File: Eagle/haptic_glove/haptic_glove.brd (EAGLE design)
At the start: 100 x 80 mm, 58 parts, among them U1 DRV2605L, U2 DRV2605L, U3 DRV2605L, U4 DRV2605L, U5 MPU-6050-1, U6 MCP73833, X1 TSW-121-07-G-S, X2 TSW-121-07-G-S, X3 TSW-121-07-G-S, X4 TSW-121-07-G-S

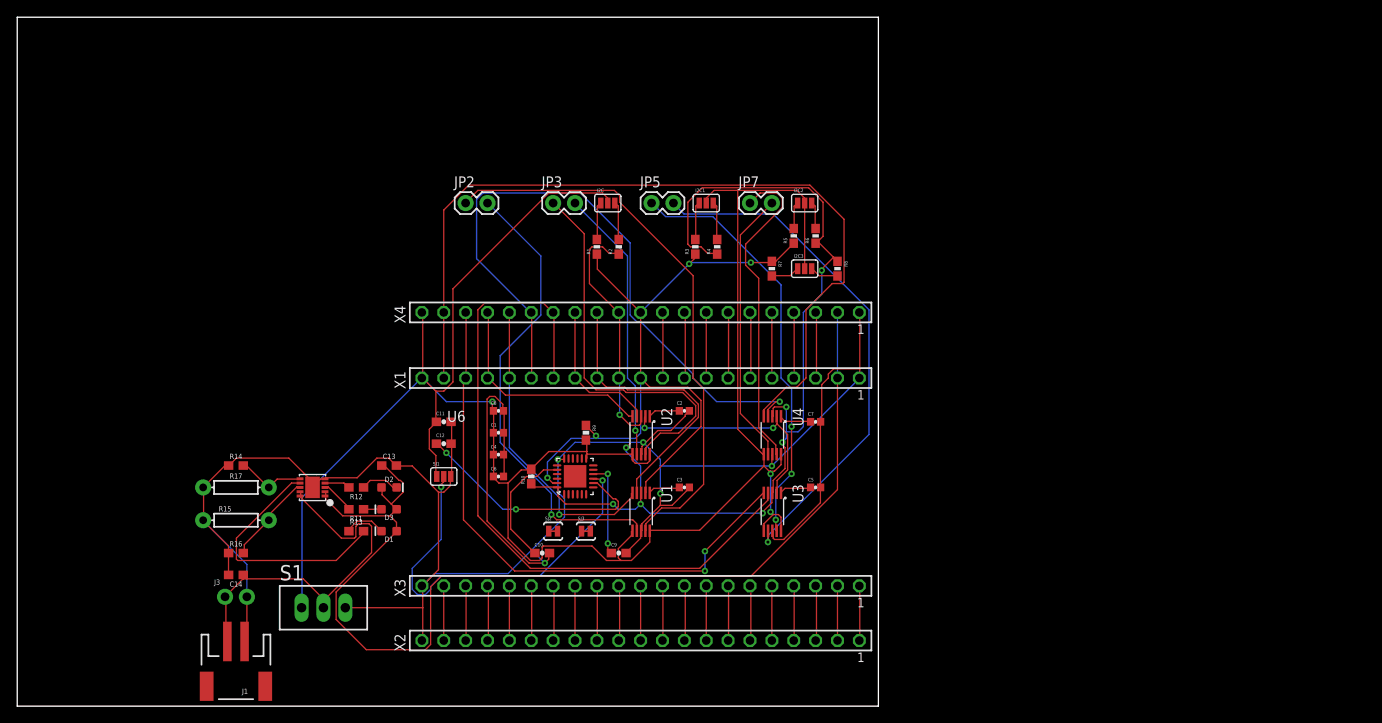
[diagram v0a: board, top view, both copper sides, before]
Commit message: Updated schematic and board design
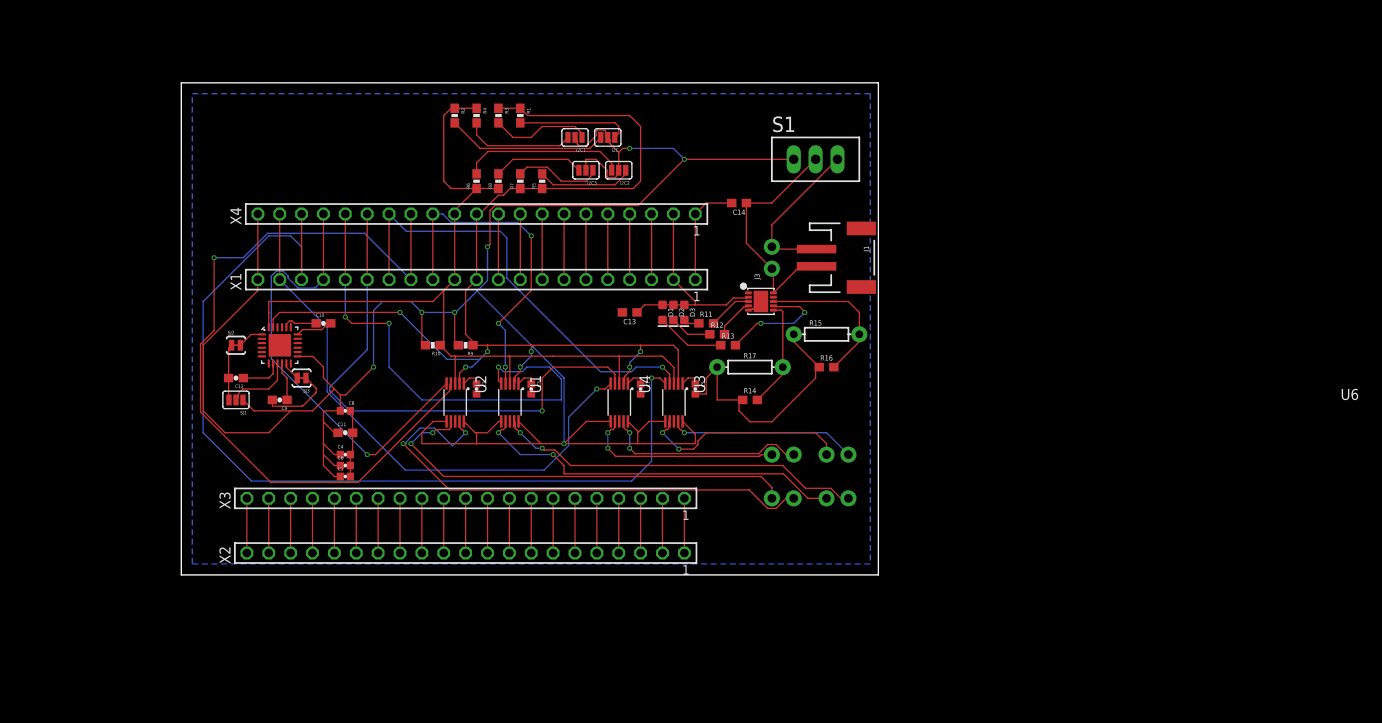
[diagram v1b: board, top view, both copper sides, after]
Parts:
- moved J1 85.9 mm to (96.5, 52.1), turned to 270 degrees
- moved S1 77.3 mm to (92.7, 63.5)
- moved J3 74.1 mm to (87.6, 50.8), turned to 90 degrees
- moved C14 72.6 mm to (83.8, 58.4)
- moved R15 71.9 mm to (94.0, 43.2)
- moved R16 71.9 mm to (94.0, 39.4)
- moved R17 61.3 mm to (85.1, 39.4)
- moved R14 60.2 mm to (85.1, 35.6)
- moved U6 56.4 mm to (86.4, 47.0), turned to 0 degrees
- moved JP2 56.1 mm to (96.5, 24.1), flipped to the bottom
- moved R13 48.3 mm to (82.5, 41.9)
- moved R11 46.0 mm to (80.0, 44.5), turned to 0 degrees
- moved R12 45.5 mm to (81.3, 43.2), turned to 0 degrees
- moved JP3 44.2 mm to (90.2, 24.1), flipped to the bottom
- moved C9 43.2 mm to (30.5, 35.6), turned to 180 degrees
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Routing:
- net GND: track 266.2 -> 97.9 mm, vias 5 -> 0
- net N$60: track 127.0 -> 25.3 mm
- net N$11: track 17.1 -> 90.1 mm, vias 0 -> 1
- net N$21: track 66.8 -> 108.6 mm, vias 2 -> 1
- net SDA: track 144.3 -> 103.5 mm, vias 8 -> 0
- net ADO: track 46.1 -> 7.99 mm, vias 2 -> 0
- net N$23: track 61.0 -> 24.5 mm, vias 1 -> 2
- net N$30: track 97.0 -> 65.7 mm, vias 0 -> 1
- net N$20: track 81.6 -> 52.2 mm, vias 0 -> 1
- net N$22: track 48.8 -> 21.8 mm, vias 3 -> 1
- net N$12: track 26.4 -> 53.2 mm, vias 0 -> 1
- net VIO: track 28.8 -> 4.86 mm, vias 2 -> 0
- net N$6: track 65.8 -> 42.9 mm, vias 0 -> 2
- net VCC: track 249.3 -> 270.5 mm, vias 3 -> 7
- net N$5: track 35.7 -> 56.8 mm, vias 1 -> 3
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- added copper zone on layer 16, net GND
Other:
- board size 100 x 80 mm -> 81 x 57.1 mm
